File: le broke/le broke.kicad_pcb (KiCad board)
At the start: 2 copper layers, 100 x 81 mm, 42 parts, among them SW1 SW_Push, U1 ProMicro

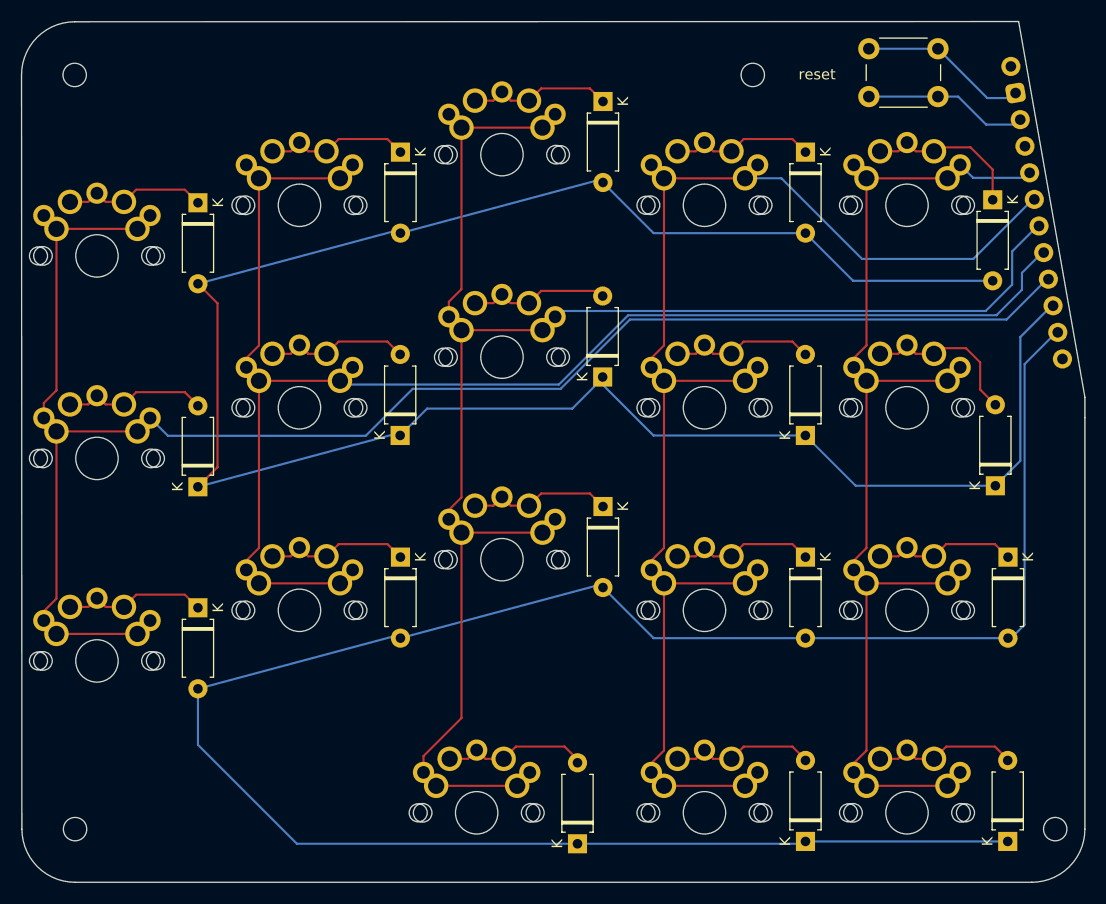
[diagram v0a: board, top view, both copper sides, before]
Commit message: a
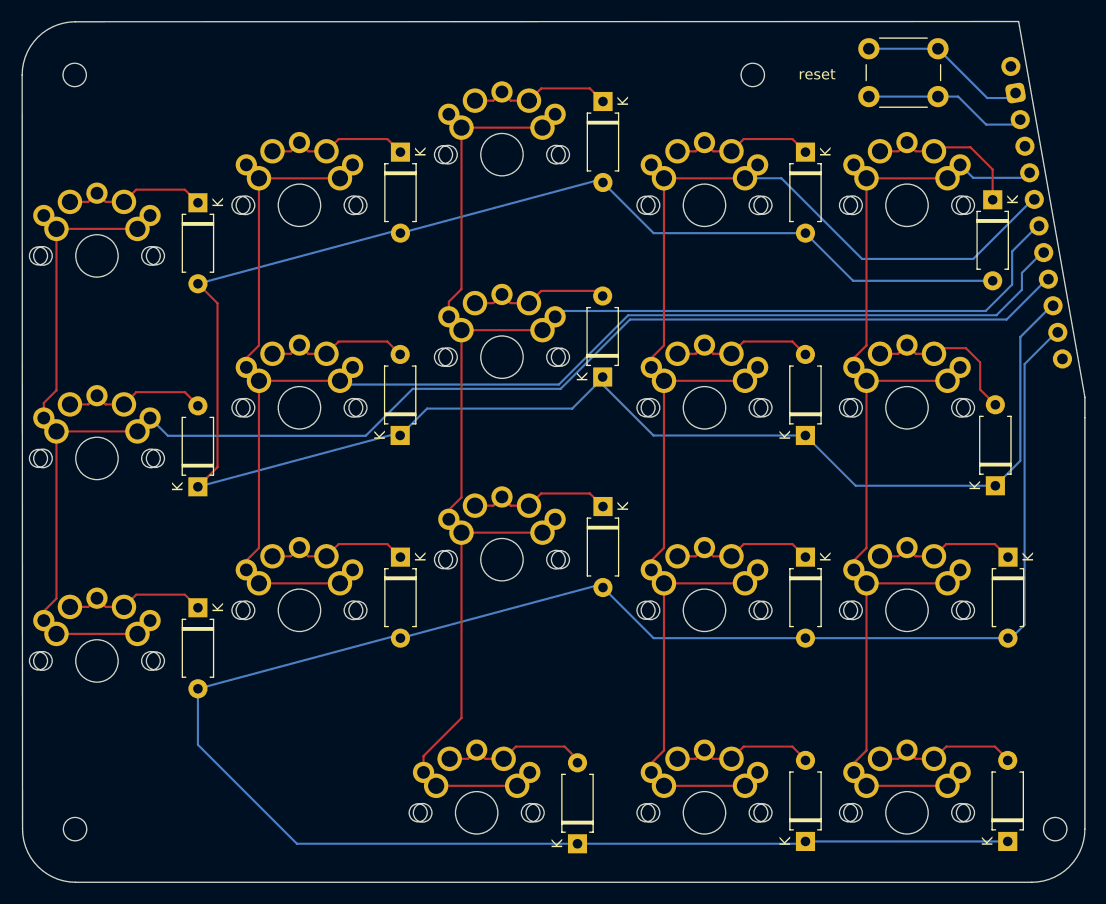
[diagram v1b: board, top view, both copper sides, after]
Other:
- outline, holes or cut-outs redrawn
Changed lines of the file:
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@@
-	)
-	(gr_line
-		(start 188.1432 131.99679)
-		(end 98.14846 131.996791)
-		(stroke
-			(width 0.05)
-			(type default)
-		)
-		(layer "Edge.Cuts")
 	)
 	(gr_line
@@
 	)
 	(gr_line
-		(start 93.112701 56.050346)
-		(end 93.148458 126.99679)
+		(start 93.172701 56.050346)
+		(end 93.208458 126.99679)
 		(stroke
 			(width 0.05)
@@
 	)
 	(gr_line
+		(start 98.208458 131.996791)
+		(end 188.1432 131.99679)
+		(stroke
+			(width 0.05)
+			(type default)
+		)
+		(layer "Edge.Cuts")
+	)
+	(gr_line
 		(start 186.91049 51.026352)
 		(end 193.143191 86.369326)
@@
 	)
 	(gr_arc
-		(start 93.112701 56.050346)
-		(mid 94.577167 52.514812)
-		(end 98.112701 51.050346)
+		(start 93.172701 56.050346)
+		(mid 94.637169 52.514815)
+		(end 98.172701 51.050346)
+		(stroke
+			(width 0.05)
+			(type default)
+		)
+		(layer "Edge.Cuts")
+	)
+	(gr_line
+		(start 186.57049 51.026444)
+		(end 98.172701 51.050363)
 		(stroke
 			(width 0.05)
@@
 	)
 	(gr_arc
-		(start 98.148458 131.996791)
-		(mid 94.612924 130.532325)
-		(end 93.148458 126.996791)
+		(start 98.208458 131.996791)
+		(mid 94.672954 130.53231)
+		(end 93.208458 126.996791)
 		(stroke
 			(width 0.05)
-			(type default)
-		)
-		(layer "Edge.Cuts")
-	)
-	(gr_line
-		(start 98.112701 51.050346)
-		(end 186.57049 51.026444)
-		(stroke
-			(width 0.05)
